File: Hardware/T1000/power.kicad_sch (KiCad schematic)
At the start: 35 parts, among them J1 USB_C_Receptacle_USB2.0, J2 Conn_01x01_Male, J3 Conn_01x01_Male, J4 Conn_01x01_Male, J5 Conn_01x01_Male, U4 LTC4419, U7 MAX77857, U8 LT6703CDC-3

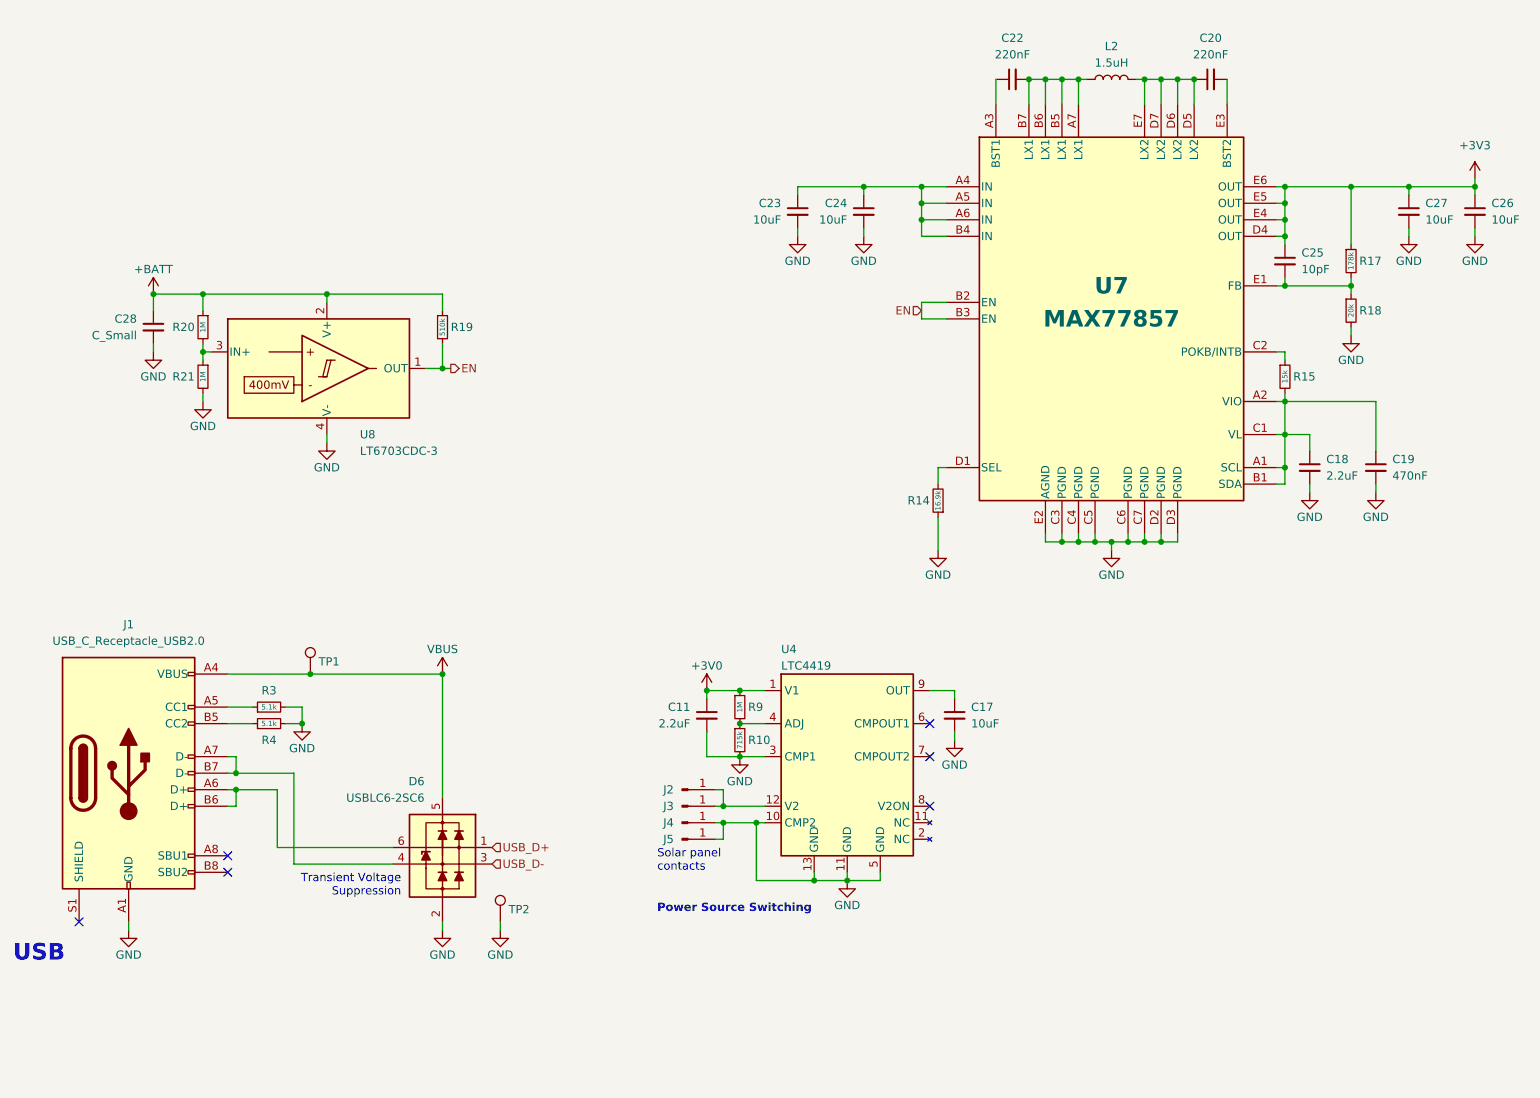
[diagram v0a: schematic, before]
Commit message: schematic updates
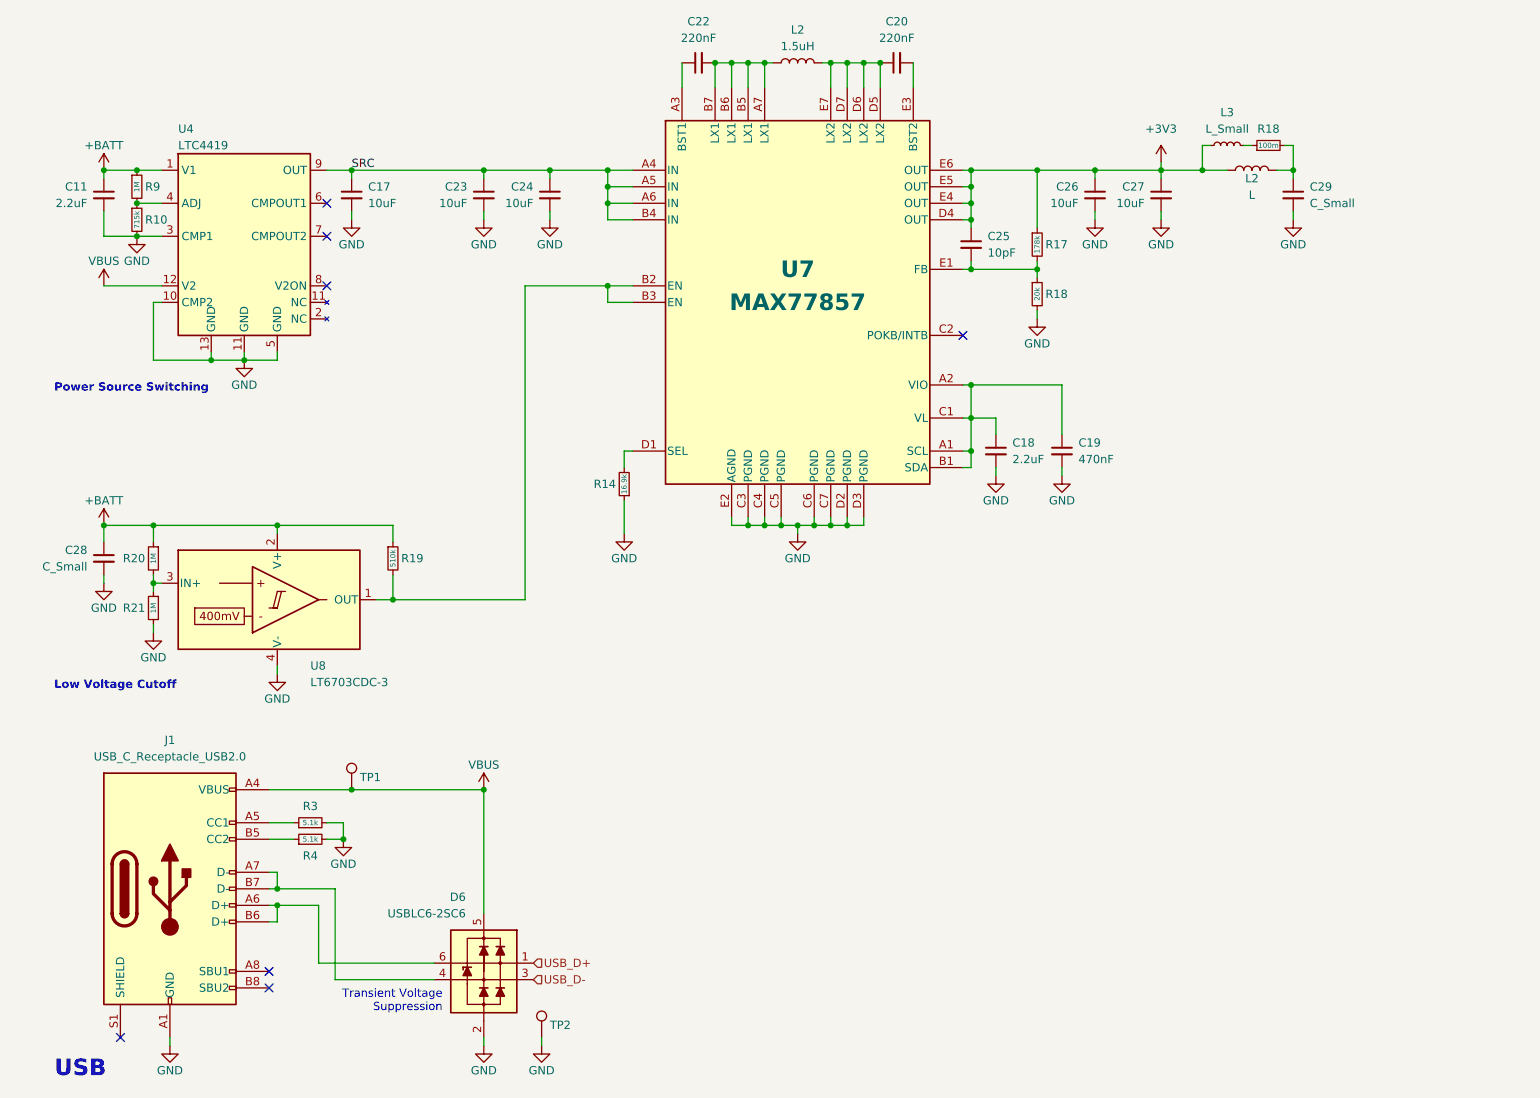
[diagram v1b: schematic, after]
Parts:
- removed J2, J3, J4, J5: Conn_01x01_Male, Connector:P19-1121, symbol Connector:Conn_01x01_Male
- removed R15: 15k, symbol Device:R_Small
- added C29: C_Small, symbol Device:C_Small
- added L2: L, symbol Device:L
- added L3: L_Small, symbol Device:L_Small
- added R18: 100m, symbol Device:R_Small
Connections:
- net +3V0 is gone; now on net +BATT: C11.1, R9.1, U4.1 (V1)
- net +3V3: now also L2.1, L3.1
- net GND: now also C29.2
- net VBUS: now also U4.12 (V2)
- net SRC: now reaches C17.1, U4.9 (OUT)
- net SRC: now also C23.1, C24.1, U7.A4 (IN), U7.A5 (IN), U7.A6 (IN), U7.B4 (IN)
- net EN: no longer names the net of R19.2, U7.B2 (EN), U7.B3 (EN), U8.1 (OUT)
- new net: C29.1, L2.2, R18.2
- new net: L3.2, R18.1
- no-connect marks 6 -> 7
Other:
- note added: "Low Voltage Cutoff"
- note removed: "Solar panel contacts"
- company: (none) -> BPP
- title: (none) -> Terminator Power System
- moved on the sheet: C11, C17, C18, C19, C20, C22, C23, C24, C25, C26, C27, C28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
